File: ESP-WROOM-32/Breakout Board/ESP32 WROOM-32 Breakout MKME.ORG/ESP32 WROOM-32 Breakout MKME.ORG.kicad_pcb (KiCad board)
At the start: 2 copper layers, 5 parts, among them J1 Screw_Terminal_01x15, J2 Screw_Terminal_01x15, J3 Conn_01x15_Female, J4 Conn_01x15_Female, U1 ESP32_DevKit_V1_DOIT

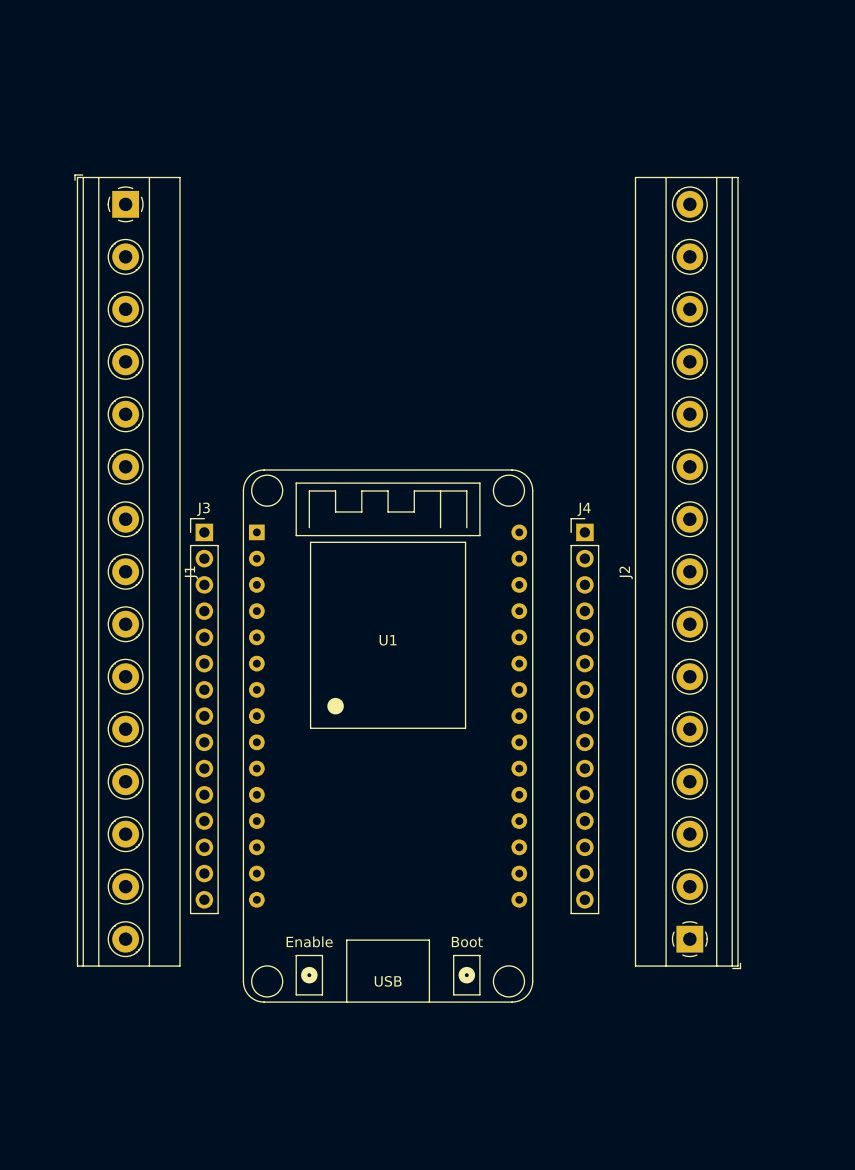
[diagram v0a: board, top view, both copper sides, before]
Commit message: Breakout board DONE
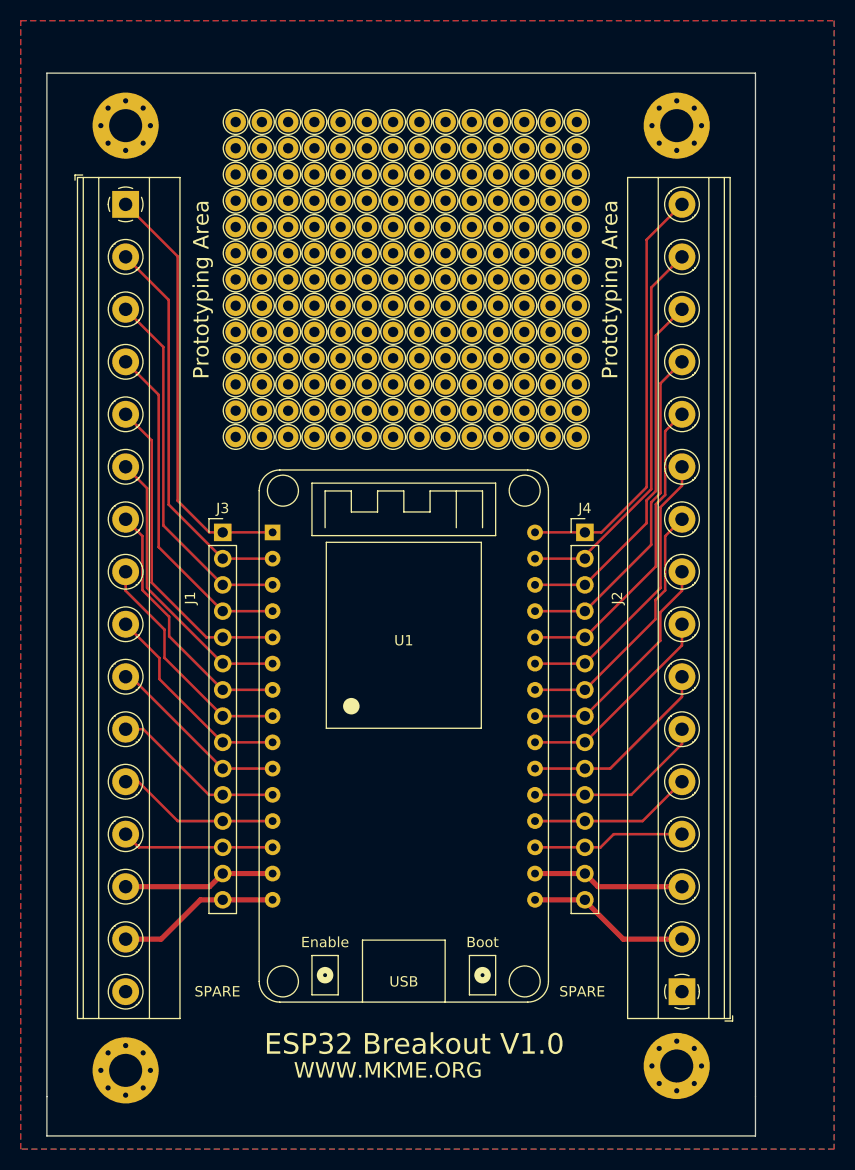
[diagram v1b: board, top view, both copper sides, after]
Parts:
- added REF**: TestPoint_THTPad_D2.0mm_Drill1.0mm, TestPoint:TestPoint_THTPad_D2.0mm_Drill1.0mm, F.Cu at (163.1, 63.1)
- added REF**: TestPoint_THTPad_D2.0mm_Drill1.0mm, TestPoint:TestPoint_THTPad_D2.0mm_Drill1.0mm, F.Cu at (140.2, 63.1)
- added REF**: TestPoint_THTPad_D2.0mm_Drill1.0mm, TestPoint:TestPoint_THTPad_D2.0mm_Drill1.0mm, F.Cu at (160.5, 45.4)
- added REF**: TestPoint_THTPad_D2.0mm_Drill1.0mm, TestPoint:TestPoint_THTPad_D2.0mm_Drill1.0mm, F.Cu at (158.0, 45.4)
- added REF**: TestPoint_THTPad_D2.0mm_Drill1.0mm, TestPoint:TestPoint_THTPad_D2.0mm_Drill1.0mm, F.Cu at (155.4, 45.4)
- added REF**: TestPoint_THTPad_D2.0mm_Drill1.0mm, TestPoint:TestPoint_THTPad_D2.0mm_Drill1.0mm, F.Cu at (152.9, 45.4)
- added REF**: TestPoint_THTPad_D2.0mm_Drill1.0mm, TestPoint:TestPoint_THTPad_D2.0mm_Drill1.0mm, F.Cu at (150.3, 45.4)
- added REF**: TestPoint_THTPad_D2.0mm_Drill1.0mm, TestPoint:TestPoint_THTPad_D2.0mm_Drill1.0mm, F.Cu at (147.8, 45.4)
- added REF**: TestPoint_THTPad_D2.0mm_Drill1.0mm, TestPoint:TestPoint_THTPad_D2.0mm_Drill1.0mm, F.Cu at (145.3, 45.4)
- added REF**: TestPoint_THTPad_D2.0mm_Drill1.0mm, TestPoint:TestPoint_THTPad_D2.0mm_Drill1.0mm, F.Cu at (142.7, 45.4)
- added REF**: TestPoint_THTPad_D2.0mm_Drill1.0mm, TestPoint:TestPoint_THTPad_D2.0mm_Drill1.0mm, F.Cu at (140.2, 45.4)
- added REF**: TestPoint_THTPad_D2.0mm_Drill1.0mm, TestPoint:TestPoint_THTPad_D2.0mm_Drill1.0mm, F.Cu at (137.7, 45.4)
- added REF**: TestPoint_THTPad_D2.0mm_Drill1.0mm, TestPoint:TestPoint_THTPad_D2.0mm_Drill1.0mm, F.Cu at (137.7, 63.1)
- added REF**: TestPoint_THTPad_D2.0mm_Drill1.0mm, TestPoint:TestPoint_THTPad_D2.0mm_Drill1.0mm, F.Cu at (135.1, 45.4)
- added REF**: TestPoint_THTPad_D2.0mm_Drill1.0mm, TestPoint:TestPoint_THTPad_D2.0mm_Drill1.0mm, F.Cu at (132.6, 45.4)
- added REF**: TestPoint_THTPad_D2.0mm_Drill1.0mm, TestPoint:TestPoint_THTPad_D2.0mm_Drill1.0mm, F.Cu at (130.0, 45.4)
- added REF**: TestPoint_THTPad_D2.0mm_Drill1.0mm, TestPoint:TestPoint_THTPad_D2.0mm_Drill1.0mm, F.Cu at (163.1, 42.8)
- added REF**: TestPoint_THTPad_D2.0mm_Drill1.0mm, TestPoint:TestPoint_THTPad_D2.0mm_Drill1.0mm, F.Cu at (160.5, 42.8)
- added REF**: TestPoint_THTPad_D2.0mm_Drill1.0mm, TestPoint:TestPoint_THTPad_D2.0mm_Drill1.0mm, F.Cu at (158.0, 42.8)
- added REF**: TestPoint_THTPad_D2.0mm_Drill1.0mm, TestPoint:TestPoint_THTPad_D2.0mm_Drill1.0mm, F.Cu at (155.4, 42.8)
- added REF**: TestPoint_THTPad_D2.0mm_Drill1.0mm, TestPoint:TestPoint_THTPad_D2.0mm_Drill1.0mm, F.Cu at (152.9, 42.8)
- added REF**: TestPoint_THTPad_D2.0mm_Drill1.0mm, TestPoint:TestPoint_THTPad_D2.0mm_Drill1.0mm, F.Cu at (150.3, 42.8)
- added REF**: TestPoint_THTPad_D2.0mm_Drill1.0mm, TestPoint:TestPoint_THTPad_D2.0mm_Drill1.0mm, F.Cu at (147.8, 42.8)
- added REF**: TestPoint_THTPad_D2.0mm_Drill1.0mm, TestPoint:TestPoint_THTPad_D2.0mm_Drill1.0mm, F.Cu at (135.1, 63.1)
- added REF**: TestPoint_THTPad_D2.0mm_Drill1.0mm, TestPoint:TestPoint_THTPad_D2.0mm_Drill1.0mm, F.Cu at (145.3, 42.8)
- added REF**: TestPoint_THTPad_D2.0mm_Drill1.0mm, TestPoint:TestPoint_THTPad_D2.0mm_Drill1.0mm, F.Cu at (142.7, 42.8)
- added REF**: TestPoint_THTPad_D2.0mm_Drill1.0mm, TestPoint:TestPoint_THTPad_D2.0mm_Drill1.0mm, F.Cu at (140.2, 42.8)
- added REF**: TestPoint_THTPad_D2.0mm_Drill1.0mm, TestPoint:TestPoint_THTPad_D2.0mm_Drill1.0mm, F.Cu at (137.7, 42.8)
- added REF**: TestPoint_THTPad_D2.0mm_Drill1.0mm, TestPoint:TestPoint_THTPad_D2.0mm_Drill1.0mm, F.Cu at (135.1, 42.8)
- added REF**: TestPoint_THTPad_D2.0mm_Drill1.0mm, TestPoint:TestPoint_THTPad_D2.0mm_Drill1.0mm, F.Cu at (132.6, 42.8)
- added REF**: TestPoint_THTPad_D2.0mm_Drill1.0mm, TestPoint:TestPoint_THTPad_D2.0mm_Drill1.0mm, F.Cu at (130.0, 42.8)
- added REF**: TestPoint_THTPad_D2.0mm_Drill1.0mm, TestPoint:TestPoint_THTPad_D2.0mm_Drill1.0mm, F.Cu at (163.1, 40.3)
- added REF**: TestPoint_THTPad_D2.0mm_Drill1.0mm, TestPoint:TestPoint_THTPad_D2.0mm_Drill1.0mm, F.Cu at (160.5, 40.3)
- added REF**: TestPoint_THTPad_D2.0mm_Drill1.0mm, TestPoint:TestPoint_THTPad_D2.0mm_Drill1.0mm, F.Cu at (158.0, 40.3)
- added REF**: TestPoint_THTPad_D2.0mm_Drill1.0mm, TestPoint:TestPoint_THTPad_D2.0mm_Drill1.0mm, F.Cu at (132.6, 63.1)
- added REF**: TestPoint_THTPad_D2.0mm_Drill1.0mm, TestPoint:TestPoint_THTPad_D2.0mm_Drill1.0mm, F.Cu at (155.4, 40.3)
- added REF**: TestPoint_THTPad_D2.0mm_Drill1.0mm, TestPoint:TestPoint_THTPad_D2.0mm_Drill1.0mm, F.Cu at (152.9, 40.3)
- added REF**: TestPoint_THTPad_D2.0mm_Drill1.0mm, TestPoint:TestPoint_THTPad_D2.0mm_Drill1.0mm, F.Cu at (150.3, 40.3)
- added REF**: TestPoint_THTPad_D2.0mm_Drill1.0mm, TestPoint:TestPoint_THTPad_D2.0mm_Drill1.0mm, F.Cu at (147.8, 40.3)
- added REF**: TestPoint_THTPad_D2.0mm_Drill1.0mm, TestPoint:TestPoint_THTPad_D2.0mm_Drill1.0mm, F.Cu at (145.3, 40.3)
- added REF**: TestPoint_THTPad_D2.0mm_Drill1.0mm, TestPoint:TestPoint_THTPad_D2.0mm_Drill1.0mm, F.Cu at (142.7, 40.3)
- added REF**: TestPoint_THTPad_D2.0mm_Drill1.0mm, TestPoint:TestPoint_THTPad_D2.0mm_Drill1.0mm, F.Cu at (140.2, 40.3)
- added REF**: TestPoint_THTPad_D2.0mm_Drill1.0mm, TestPoint:TestPoint_THTPad_D2.0mm_Drill1.0mm, F.Cu at (137.7, 40.3)
- added REF**: TestPoint_THTPad_D2.0mm_Drill1.0mm, TestPoint:TestPoint_THTPad_D2.0mm_Drill1.0mm, F.Cu at (135.1, 40.3)
- added REF**: TestPoint_THTPad_D2.0mm_Drill1.0mm, TestPoint:TestPoint_THTPad_D2.0mm_Drill1.0mm, F.Cu at (132.6, 40.3)
- added REF**: TestPoint_THTPad_D2.0mm_Drill1.0mm, TestPoint:TestPoint_THTPad_D2.0mm_Drill1.0mm, F.Cu at (130.0, 63.1)
- added REF**: TestPoint_THTPad_D2.0mm_Drill1.0mm, TestPoint:TestPoint_THTPad_D2.0mm_Drill1.0mm, F.Cu at (130.0, 40.3)
- added REF**: TestPoint_THTPad_D2.0mm_Drill1.0mm, TestPoint:TestPoint_THTPad_D2.0mm_Drill1.0mm, F.Cu at (163.1, 37.8)
- added REF**: TestPoint_THTPad_D2.0mm_Drill1.0mm, TestPoint:TestPoint_THTPad_D2.0mm_Drill1.0mm, F.Cu at (160.5, 37.8)
- added REF**: TestPoint_THTPad_D2.0mm_Drill1.0mm, TestPoint:TestPoint_THTPad_D2.0mm_Drill1.0mm, F.Cu at (158.0, 37.8)
- added REF**: TestPoint_THTPad_D2.0mm_Drill1.0mm, TestPoint:TestPoint_THTPad_D2.0mm_Drill1.0mm, F.Cu at (155.4, 37.8)
- added REF**: TestPoint_THTPad_D2.0mm_Drill1.0mm, TestPoint:TestPoint_THTPad_D2.0mm_Drill1.0mm, F.Cu at (152.9, 37.8)
- added REF**: TestPoint_THTPad_D2.0mm_Drill1.0mm, TestPoint:TestPoint_THTPad_D2.0mm_Drill1.0mm, F.Cu at (150.3, 37.8)
- added REF**: TestPoint_THTPad_D2.0mm_Drill1.0mm, TestPoint:TestPoint_THTPad_D2.0mm_Drill1.0mm, F.Cu at (147.8, 37.8)
- added REF**: TestPoint_THTPad_D2.0mm_Drill1.0mm, TestPoint:TestPoint_THTPad_D2.0mm_Drill1.0mm, F.Cu at (145.3, 37.8)
- added REF**: TestPoint_THTPad_D2.0mm_Drill1.0mm, TestPoint:TestPoint_THTPad_D2.0mm_Drill1.0mm, F.Cu at (142.7, 37.8)
- added REF**: TestPoint_THTPad_D2.0mm_Drill1.0mm, TestPoint:TestPoint_THTPad_D2.0mm_Drill1.0mm, F.Cu at (163.1, 60.6)
- added REF**: TestPoint_THTPad_D2.0mm_Drill1.0mm, TestPoint:TestPoint_THTPad_D2.0mm_Drill1.0mm, F.Cu at (140.2, 37.8)
- added REF**: TestPoint_THTPad_D2.0mm_Drill1.0mm, TestPoint:TestPoint_THTPad_D2.0mm_Drill1.0mm, F.Cu at (137.7, 37.8)
- added REF**: TestPoint_THTPad_D2.0mm_Drill1.0mm, TestPoint:TestPoint_THTPad_D2.0mm_Drill1.0mm, F.Cu at (135.1, 37.8)
- added REF**: TestPoint_THTPad_D2.0mm_Drill1.0mm, TestPoint:TestPoint_THTPad_D2.0mm_Drill1.0mm, F.Cu at (132.6, 37.8)
- added REF**: TestPoint_THTPad_D2.0mm_Drill1.0mm, TestPoint:TestPoint_THTPad_D2.0mm_Drill1.0mm, F.Cu at (130.0, 37.8)
- added REF**: TestPoint_THTPad_D2.0mm_Drill1.0mm, TestPoint:TestPoint_THTPad_D2.0mm_Drill1.0mm, F.Cu at (163.1, 35.2)
- added REF**: TestPoint_THTPad_D2.0mm_Drill1.0mm, TestPoint:TestPoint_THTPad_D2.0mm_Drill1.0mm, F.Cu at (160.5, 35.2)
- added REF**: TestPoint_THTPad_D2.0mm_Drill1.0mm, TestPoint:TestPoint_THTPad_D2.0mm_Drill1.0mm, F.Cu at (158.0, 35.2)
- added REF**: TestPoint_THTPad_D2.0mm_Drill1.0mm, TestPoint:TestPoint_THTPad_D2.0mm_Drill1.0mm, F.Cu at (155.4, 35.2)
- added REF**: TestPoint_THTPad_D2.0mm_Drill1.0mm, TestPoint:TestPoint_THTPad_D2.0mm_Drill1.0mm, F.Cu at (152.9, 35.2)
- added REF**: TestPoint_THTPad_D2.0mm_Drill1.0mm, TestPoint:TestPoint_THTPad_D2.0mm_Drill1.0mm, F.Cu at (160.5, 60.6)
- added REF**: TestPoint_THTPad_D2.0mm_Drill1.0mm, TestPoint:TestPoint_THTPad_D2.0mm_Drill1.0mm, F.Cu at (150.3, 35.2)
- added REF**: TestPoint_THTPad_D2.0mm_Drill1.0mm, TestPoint:TestPoint_THTPad_D2.0mm_Drill1.0mm, F.Cu at (147.8, 35.2)
- added REF**: TestPoint_THTPad_D2.0mm_Drill1.0mm, TestPoint:TestPoint_THTPad_D2.0mm_Drill1.0mm, F.Cu at (145.3, 35.2)
- added REF**: TestPoint_THTPad_D2.0mm_Drill1.0mm, TestPoint:TestPoint_THTPad_D2.0mm_Drill1.0mm, F.Cu at (142.7, 35.2)
- added REF**: TestPoint_THTPad_D2.0mm_Drill1.0mm, TestPoint:TestPoint_THTPad_D2.0mm_Drill1.0mm, F.Cu at (140.2, 35.2)
- added REF**: TestPoint_THTPad_D2.0mm_Drill1.0mm, TestPoint:TestPoint_THTPad_D2.0mm_Drill1.0mm, F.Cu at (137.7, 35.2)
- added REF**: TestPoint_THTPad_D2.0mm_Drill1.0mm, TestPoint:TestPoint_THTPad_D2.0mm_Drill1.0mm, F.Cu at (135.1, 35.2)
- added REF**: TestPoint_THTPad_D2.0mm_Drill1.0mm, TestPoint:TestPoint_THTPad_D2.0mm_Drill1.0mm, F.Cu at (132.6, 35.2)
- added REF**: TestPoint_THTPad_D2.0mm_Drill1.0mm, TestPoint:TestPoint_THTPad_D2.0mm_Drill1.0mm, F.Cu at (130.0, 35.2)
- added REF**: TestPoint_THTPad_D2.0mm_Drill1.0mm, TestPoint:TestPoint_THTPad_D2.0mm_Drill1.0mm, F.Cu at (163.1, 32.7)
- added REF**: TestPoint_THTPad_D2.0mm_Drill1.0mm, TestPoint:TestPoint_THTPad_D2.0mm_Drill1.0mm, F.Cu at (158.0, 60.6)
- added REF**: TestPoint_THTPad_D2.0mm_Drill1.0mm, TestPoint:TestPoint_THTPad_D2.0mm_Drill1.0mm, F.Cu at (160.5, 32.7)
- added REF**: TestPoint_THTPad_D2.0mm_Drill1.0mm, TestPoint:TestPoint_THTPad_D2.0mm_Drill1.0mm, F.Cu at (158.0, 32.7)
- added REF**: TestPoint_THTPad_D2.0mm_Drill1.0mm, TestPoint:TestPoint_THTPad_D2.0mm_Drill1.0mm, F.Cu at (155.4, 32.7)
- added REF**: TestPoint_THTPad_D2.0mm_Drill1.0mm, TestPoint:TestPoint_THTPad_D2.0mm_Drill1.0mm, F.Cu at (152.9, 32.7)
- added REF**: TestPoint_THTPad_D2.0mm_Drill1.0mm, TestPoint:TestPoint_THTPad_D2.0mm_Drill1.0mm, F.Cu at (150.3, 32.7)
- added REF**: TestPoint_THTPad_D2.0mm_Drill1.0mm, TestPoint:TestPoint_THTPad_D2.0mm_Drill1.0mm, F.Cu at (147.8, 32.7)
- added REF**: TestPoint_THTPad_D2.0mm_Drill1.0mm, TestPoint:TestPoint_THTPad_D2.0mm_Drill1.0mm, F.Cu at (145.3, 32.7)
- added REF**: TestPoint_THTPad_D2.0mm_Drill1.0mm, TestPoint:TestPoint_THTPad_D2.0mm_Drill1.0mm, F.Cu at (142.7, 32.7)
- added REF**: TestPoint_THTPad_D2.0mm_Drill1.0mm, TestPoint:TestPoint_THTPad_D2.0mm_Drill1.0mm, F.Cu at (140.2, 32.7)
- added REF**: TestPoint_THTPad_D2.0mm_Drill1.0mm, TestPoint:TestPoint_THTPad_D2.0mm_Drill1.0mm, F.Cu at (137.7, 32.7)
- added REF**: TestPoint_THTPad_D2.0mm_Drill1.0mm, TestPoint:TestPoint_THTPad_D2.0mm_Drill1.0mm, F.Cu at (155.4, 60.6)
- added REF**: TestPoint_THTPad_D2.0mm_Drill1.0mm, TestPoint:TestPoint_THTPad_D2.0mm_Drill1.0mm, F.Cu at (135.1, 32.7)
- added REF**: TestPoint_THTPad_D2.0mm_Drill1.0mm, TestPoint:TestPoint_THTPad_D2.0mm_Drill1.0mm, F.Cu at (132.6, 32.7)
- added REF**: TestPoint_THTPad_D2.0mm_Drill1.0mm, TestPoint:TestPoint_THTPad_D2.0mm_Drill1.0mm, F.Cu at (130.0, 32.7)
- added REF**: MountingHole_3.2mm_M3_Pad_Via, MountingHole:MountingHole_3.2mm_M3_Pad_Via, F.Cu at (172.7, 33.0)
- added REF**: MountingHole_3.2mm_M3_Pad_Via, MountingHole:MountingHole_3.2mm_M3_Pad_Via, F.Cu at (119.4, 33.0)
- added REF**: MountingHole_3.2mm_M3_Pad_Via, MountingHole:MountingHole_3.2mm_M3_Pad_Via, F.Cu at (119.4, 124.5)
- added REF**: MountingHole_3.2mm_M3_Pad_Via, MountingHole:MountingHole_3.2mm_M3_Pad_Via, F.Cu at (172.7, 124.0)
- added REF**: TestPoint_THTPad_D2.0mm_Drill1.0mm, TestPoint:TestPoint_THTPad_D2.0mm_Drill1.0mm, F.Cu at (152.9, 60.6)
- added REF**: TestPoint_THTPad_D2.0mm_Drill1.0mm, TestPoint:TestPoint_THTPad_D2.0mm_Drill1.0mm, F.Cu at (160.5, 63.1)
- added REF**: TestPoint_THTPad_D2.0mm_Drill1.0mm, TestPoint:TestPoint_THTPad_D2.0mm_Drill1.0mm, F.Cu at (150.3, 60.6)
- added REF**: TestPoint_THTPad_D2.0mm_Drill1.0mm, TestPoint:TestPoint_THTPad_D2.0mm_Drill1.0mm, F.Cu at (147.8, 60.6)
- added REF**: TestPoint_THTPad_D2.0mm_Drill1.0mm, TestPoint:TestPoint_THTPad_D2.0mm_Drill1.0mm, F.Cu at (145.3, 60.6)
- added REF**: TestPoint_THTPad_D2.0mm_Drill1.0mm, TestPoint:TestPoint_THTPad_D2.0mm_Drill1.0mm, F.Cu at (142.7, 60.6)
- added REF**: TestPoint_THTPad_D2.0mm_Drill1.0mm, TestPoint:TestPoint_THTPad_D2.0mm_Drill1.0mm, F.Cu at (140.2, 60.6)
- added REF**: TestPoint_THTPad_D2.0mm_Drill1.0mm, TestPoint:TestPoint_THTPad_D2.0mm_Drill1.0mm, F.Cu at (137.7, 60.6)
- added REF**: TestPoint_THTPad_D2.0mm_Drill1.0mm, TestPoint:TestPoint_THTPad_D2.0mm_Drill1.0mm, F.Cu at (135.1, 60.6)
- added REF**: TestPoint_THTPad_D2.0mm_Drill1.0mm, TestPoint:TestPoint_THTPad_D2.0mm_Drill1.0mm, F.Cu at (132.6, 60.6)
- added REF**: TestPoint_THTPad_D2.0mm_Drill1.0mm, TestPoint:TestPoint_THTPad_D2.0mm_Drill1.0mm, F.Cu at (130.0, 60.6)
- added REF**: TestPoint_THTPad_D2.0mm_Drill1.0mm, TestPoint:TestPoint_THTPad_D2.0mm_Drill1.0mm, F.Cu at (163.1, 58.1)
- added REF**: TestPoint_THTPad_D2.0mm_Drill1.0mm, TestPoint:TestPoint_THTPad_D2.0mm_Drill1.0mm, F.Cu at (158.0, 63.1)
- added REF**: TestPoint_THTPad_D2.0mm_Drill1.0mm, TestPoint:TestPoint_THTPad_D2.0mm_Drill1.0mm, F.Cu at (160.5, 58.1)
- added REF**: TestPoint_THTPad_D2.0mm_Drill1.0mm, TestPoint:TestPoint_THTPad_D2.0mm_Drill1.0mm, F.Cu at (158.0, 58.1)
- added REF**: TestPoint_THTPad_D2.0mm_Drill1.0mm, TestPoint:TestPoint_THTPad_D2.0mm_Drill1.0mm, F.Cu at (155.4, 58.1)
- added REF**: TestPoint_THTPad_D2.0mm_Drill1.0mm, TestPoint:TestPoint_THTPad_D2.0mm_Drill1.0mm, F.Cu at (152.9, 58.1)
- added REF**: TestPoint_THTPad_D2.0mm_Drill1.0mm, TestPoint:TestPoint_THTPad_D2.0mm_Drill1.0mm, F.Cu at (150.3, 58.1)
- added REF**: TestPoint_THTPad_D2.0mm_Drill1.0mm, TestPoint:TestPoint_THTPad_D2.0mm_Drill1.0mm, F.Cu at (147.8, 58.1)
- added REF**: TestPoint_THTPad_D2.0mm_Drill1.0mm, TestPoint:TestPoint_THTPad_D2.0mm_Drill1.0mm, F.Cu at (145.3, 58.1)
- added REF**: TestPoint_THTPad_D2.0mm_Drill1.0mm, TestPoint:TestPoint_THTPad_D2.0mm_Drill1.0mm, F.Cu at (142.7, 58.1)
- added REF**: TestPoint_THTPad_D2.0mm_Drill1.0mm, TestPoint:TestPoint_THTPad_D2.0mm_Drill1.0mm, F.Cu at (140.2, 58.1)
- added REF**: TestPoint_THTPad_D2.0mm_Drill1.0mm, TestPoint:TestPoint_THTPad_D2.0mm_Drill1.0mm, F.Cu at (137.7, 58.1)
- added REF**: TestPoint_THTPad_D2.0mm_Drill1.0mm, TestPoint:TestPoint_THTPad_D2.0mm_Drill1.0mm, F.Cu at (155.4, 63.1)
- added REF**: TestPoint_THTPad_D2.0mm_Drill1.0mm, TestPoint:TestPoint_THTPad_D2.0mm_Drill1.0mm, F.Cu at (135.1, 58.1)
- added REF**: TestPoint_THTPad_D2.0mm_Drill1.0mm, TestPoint:TestPoint_THTPad_D2.0mm_Drill1.0mm, F.Cu at (132.6, 58.1)
- added REF**: TestPoint_THTPad_D2.0mm_Drill1.0mm, TestPoint:TestPoint_THTPad_D2.0mm_Drill1.0mm, F.Cu at (130.0, 58.1)
- added REF**: TestPoint_THTPad_D2.0mm_Drill1.0mm, TestPoint:TestPoint_THTPad_D2.0mm_Drill1.0mm, F.Cu at (163.1, 55.5)
- added REF**: TestPoint_THTPad_D2.0mm_Drill1.0mm, TestPoint:TestPoint_THTPad_D2.0mm_Drill1.0mm, F.Cu at (160.5, 55.5)
- added REF**: TestPoint_THTPad_D2.0mm_Drill1.0mm, TestPoint:TestPoint_THTPad_D2.0mm_Drill1.0mm, F.Cu at (158.0, 55.5)
- added REF**: TestPoint_THTPad_D2.0mm_Drill1.0mm, TestPoint:TestPoint_THTPad_D2.0mm_Drill1.0mm, F.Cu at (155.4, 55.5)
- added REF**: TestPoint_THTPad_D2.0mm_Drill1.0mm, TestPoint:TestPoint_THTPad_D2.0mm_Drill1.0mm, F.Cu at (152.9, 55.5)
- added REF**: TestPoint_THTPad_D2.0mm_Drill1.0mm, TestPoint:TestPoint_THTPad_D2.0mm_Drill1.0mm, F.Cu at (150.3, 55.5)
- added REF**: TestPoint_THTPad_D2.0mm_Drill1.0mm, TestPoint:TestPoint_THTPad_D2.0mm_Drill1.0mm, F.Cu at (147.8, 55.5)
- added REF**: TestPoint_THTPad_D2.0mm_Drill1.0mm, TestPoint:TestPoint_THTPad_D2.0mm_Drill1.0mm, F.Cu at (152.9, 63.1)
- added REF**: TestPoint_THTPad_D2.0mm_Drill1.0mm, TestPoint:TestPoint_THTPad_D2.0mm_Drill1.0mm, F.Cu at (145.3, 55.5)
- added REF**: TestPoint_THTPad_D2.0mm_Drill1.0mm, TestPoint:TestPoint_THTPad_D2.0mm_Drill1.0mm, F.Cu at (142.7, 55.5)
- added REF**: TestPoint_THTPad_D2.0mm_Drill1.0mm, TestPoint:TestPoint_THTPad_D2.0mm_Drill1.0mm, F.Cu at (140.2, 55.5)
- added REF**: TestPoint_THTPad_D2.0mm_Drill1.0mm, TestPoint:TestPoint_THTPad_D2.0mm_Drill1.0mm, F.Cu at (137.7, 55.5)
- added REF**: TestPoint_THTPad_D2.0mm_Drill1.0mm, TestPoint:TestPoint_THTPad_D2.0mm_Drill1.0mm, F.Cu at (135.1, 55.5)
- added REF**: TestPoint_THTPad_D2.0mm_Drill1.0mm, TestPoint:TestPoint_THTPad_D2.0mm_Drill1.0mm, F.Cu at (132.6, 55.5)
- added REF**: TestPoint_THTPad_D2.0mm_Drill1.0mm, TestPoint:TestPoint_THTPad_D2.0mm_Drill1.0mm, F.Cu at (130.0, 55.5)
- added REF**: TestPoint_THTPad_D2.0mm_Drill1.0mm, TestPoint:TestPoint_THTPad_D2.0mm_Drill1.0mm, F.Cu at (163.1, 53.0)
- added REF**: TestPoint_THTPad_D2.0mm_Drill1.0mm, TestPoint:TestPoint_THTPad_D2.0mm_Drill1.0mm, F.Cu at (160.5, 53.0)
- added REF**: TestPoint_THTPad_D2.0mm_Drill1.0mm, TestPoint:TestPoint_THTPad_D2.0mm_Drill1.0mm, F.Cu at (158.0, 53.0)
- added REF**: TestPoint_THTPad_D2.0mm_Drill1.0mm, TestPoint:TestPoint_THTPad_D2.0mm_Drill1.0mm, F.Cu at (150.3, 63.1)
- added REF**: TestPoint_THTPad_D2.0mm_Drill1.0mm, TestPoint:TestPoint_THTPad_D2.0mm_Drill1.0mm, F.Cu at (155.4, 53.0)
- added REF**: TestPoint_THTPad_D2.0mm_Drill1.0mm, TestPoint:TestPoint_THTPad_D2.0mm_Drill1.0mm, F.Cu at (152.9, 53.0)
- added REF**: TestPoint_THTPad_D2.0mm_Drill1.0mm, TestPoint:TestPoint_THTPad_D2.0mm_Drill1.0mm, F.Cu at (150.3, 53.0)
- added REF**: TestPoint_THTPad_D2.0mm_Drill1.0mm, TestPoint:TestPoint_THTPad_D2.0mm_Drill1.0mm, F.Cu at (147.8, 53.0)
- added REF**: TestPoint_THTPad_D2.0mm_Drill1.0mm, TestPoint:TestPoint_THTPad_D2.0mm_Drill1.0mm, F.Cu at (145.3, 53.0)
- added REF**: TestPoint_THTPad_D2.0mm_Drill1.0mm, TestPoint:TestPoint_THTPad_D2.0mm_Drill1.0mm, F.Cu at (142.7, 53.0)
- added REF**: TestPoint_THTPad_D2.0mm_Drill1.0mm, TestPoint:TestPoint_THTPad_D2.0mm_Drill1.0mm, F.Cu at (140.2, 53.0)
- added REF**: TestPoint_THTPad_D2.0mm_Drill1.0mm, TestPoint:TestPoint_THTPad_D2.0mm_Drill1.0mm, F.Cu at (137.7, 53.0)
- added REF**: TestPoint_THTPad_D2.0mm_Drill1.0mm, TestPoint:TestPoint_THTPad_D2.0mm_Drill1.0mm, F.Cu at (135.1, 53.0)
- added REF**: TestPoint_THTPad_D2.0mm_Drill1.0mm, TestPoint:TestPoint_THTPad_D2.0mm_Drill1.0mm, F.Cu at (132.6, 53.0)
- added REF**: TestPoint_THTPad_D2.0mm_Drill1.0mm, TestPoint:TestPoint_THTPad_D2.0mm_Drill1.0mm, F.Cu at (147.8, 63.1)
- added REF**: TestPoint_THTPad_D2.0mm_Drill1.0mm, TestPoint:TestPoint_THTPad_D2.0mm_Drill1.0mm, F.Cu at (130.0, 53.0)
- added REF**: TestPoint_THTPad_D2.0mm_Drill1.0mm, TestPoint:TestPoint_THTPad_D2.0mm_Drill1.0mm, F.Cu at (163.1, 50.5)
- added REF**: TestPoint_THTPad_D2.0mm_Drill1.0mm, TestPoint:TestPoint_THTPad_D2.0mm_Drill1.0mm, F.Cu at (160.5, 50.5)
- added REF**: TestPoint_THTPad_D2.0mm_Drill1.0mm, TestPoint:TestPoint_THTPad_D2.0mm_Drill1.0mm, F.Cu at (158.0, 50.5)
- added REF**: TestPoint_THTPad_D2.0mm_Drill1.0mm, TestPoint:TestPoint_THTPad_D2.0mm_Drill1.0mm, F.Cu at (155.4, 50.5)
- added REF**: TestPoint_THTPad_D2.0mm_Drill1.0mm, TestPoint:TestPoint_THTPad_D2.0mm_Drill1.0mm, F.Cu at (152.9, 50.5)
- added REF**: TestPoint_THTPad_D2.0mm_Drill1.0mm, TestPoint:TestPoint_THTPad_D2.0mm_Drill1.0mm, F.Cu at (150.3, 50.5)
- added REF**: TestPoint_THTPad_D2.0mm_Drill1.0mm, TestPoint:TestPoint_THTPad_D2.0mm_Drill1.0mm, F.Cu at (147.8, 50.5)
- added REF**: TestPoint_THTPad_D2.0mm_Drill1.0mm, TestPoint:TestPoint_THTPad_D2.0mm_Drill1.0mm, F.Cu at (145.3, 50.5)
- added REF**: TestPoint_THTPad_D2.0mm_Drill1.0mm, TestPoint:TestPoint_THTPad_D2.0mm_Drill1.0mm, F.Cu at (142.7, 50.5)
- added REF**: TestPoint_THTPad_D2.0mm_Drill1.0mm, TestPoint:TestPoint_THTPad_D2.0mm_Drill1.0mm, F.Cu at (145.3, 63.1)
- added REF**: TestPoint_THTPad_D2.0mm_Drill1.0mm, TestPoint:TestPoint_THTPad_D2.0mm_Drill1.0mm, F.Cu at (140.2, 50.5)
- added REF**: TestPoint_THTPad_D2.0mm_Drill1.0mm, TestPoint:TestPoint_THTPad_D2.0mm_Drill1.0mm, F.Cu at (137.7, 50.5)
- added REF**: TestPoint_THTPad_D2.0mm_Drill1.0mm, TestPoint:TestPoint_THTPad_D2.0mm_Drill1.0mm, F.Cu at (135.1, 50.5)
- added REF**: TestPoint_THTPad_D2.0mm_Drill1.0mm, TestPoint:TestPoint_THTPad_D2.0mm_Drill1.0mm, F.Cu at (132.6, 50.5)
- added REF**: TestPoint_THTPad_D2.0mm_Drill1.0mm, TestPoint:TestPoint_THTPad_D2.0mm_Drill1.0mm, F.Cu at (130.0, 50.5)
- added REF**: TestPoint_THTPad_D2.0mm_Drill1.0mm, TestPoint:TestPoint_THTPad_D2.0mm_Drill1.0mm, F.Cu at (163.1, 47.9)
- added REF**: TestPoint_THTPad_D2.0mm_Drill1.0mm, TestPoint:TestPoint_THTPad_D2.0mm_Drill1.0mm, F.Cu at (160.5, 47.9)
- added REF**: TestPoint_THTPad_D2.0mm_Drill1.0mm, TestPoint:TestPoint_THTPad_D2.0mm_Drill1.0mm, F.Cu at (158.0, 47.9)
- added REF**: TestPoint_THTPad_D2.0mm_Drill1.0mm, TestPoint:TestPoint_THTPad_D2.0mm_Drill1.0mm, F.Cu at (155.4, 47.9)
- added REF**: TestPoint_THTPad_D2.0mm_Drill1.0mm, TestPoint:TestPoint_THTPad_D2.0mm_Drill1.0mm, F.Cu at (152.9, 47.9)
- added REF**: TestPoint_THTPad_D2.0mm_Drill1.0mm, TestPoint:TestPoint_THTPad_D2.0mm_Drill1.0mm, F.Cu at (142.7, 63.1)
- added REF**: TestPoint_THTPad_D2.0mm_Drill1.0mm, TestPoint:TestPoint_THTPad_D2.0mm_Drill1.0mm, F.Cu at (150.3, 47.9)
- added REF**: TestPoint_THTPad_D2.0mm_Drill1.0mm, TestPoint:TestPoint_THTPad_D2.0mm_Drill1.0mm, F.Cu at (147.8, 47.9)
- added REF**: TestPoint_THTPad_D2.0mm_Drill1.0mm, TestPoint:TestPoint_THTPad_D2.0mm_Drill1.0mm, F.Cu at (145.3, 47.9)
- added REF**: TestPoint_THTPad_D2.0mm_Drill1.0mm, TestPoint:TestPoint_THTPad_D2.0mm_Drill1.0mm, F.Cu at (142.7, 47.9)
- added REF**: TestPoint_THTPad_D2.0mm_Drill1.0mm, TestPoint:TestPoint_THTPad_D2.0mm_Drill1.0mm, F.Cu at (140.2, 47.9)
- added REF**: TestPoint_THTPad_D2.0mm_Drill1.0mm, TestPoint:TestPoint_THTPad_D2.0mm_Drill1.0mm, F.Cu at (137.7, 47.9)
- added REF**: TestPoint_THTPad_D2.0mm_Drill1.0mm, TestPoint:TestPoint_THTPad_D2.0mm_Drill1.0mm, F.Cu at (135.1, 47.9)
- added REF**: TestPoint_THTPad_D2.0mm_Drill1.0mm, TestPoint:TestPoint_THTPad_D2.0mm_Drill1.0mm, F.Cu at (132.6, 47.9)
- added REF**: TestPoint_THTPad_D2.0mm_Drill1.0mm, TestPoint:TestPoint_THTPad_D2.0mm_Drill1.0mm, F.Cu at (130.0, 47.9)
- added REF**: TestPoint_THTPad_D2.0mm_Drill1.0mm, TestPoint:TestPoint_THTPad_D2.0mm_Drill1.0mm, F.Cu at (163.1, 45.4)
- J1, J2: footprint TerminalBlock_Phoenix:TerminalBlock_Phoenix_MKDS-1,5-15-5.08_1x15_P5.08mm_Horizontal -> TerminalBlock_Phoenix:TerminalBlock_Phoenix_MKDS-1,5-16-5.08_1x16_P5.08mm_Horizontal
- moved J2 5.14 mm to (173.2, 116.8)
- moved J3 1.78 mm to (128.8, 72.4)
- moved U1 1.52 mm to (146.3, 72.4)
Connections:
- J2 pad 1: 3V3 -> Net-(J2-Pad1)
- J2 pad 10: D19 -> D18
- J2 pad 11: D21 -> D19
- J2 pad 12: RX0 -> D21
- J2 pad 13: TX0 -> RX0
- J2 pad 14: D22 -> TX0
- J2 pad 15: D23 -> D22
- J2 pad 2: GND -> 3V3
- J2 pad 3: D15 -> GND
- J2 pad 4: D2 -> D15
- J2 pad 5: D4 -> D2
- J2 pad 6: RX2 -> D4
- J2 pad 7: TX2 -> RX2
- J2 pad 8: D5 -> TX2
- J2 pad 9: D18 -> D5
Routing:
- net D23: track 0.00 -> 42.2 mm
- net EN: track 0.00 -> 41.2 mm
- net VP: track 0.00 -> 37.9 mm
- net D22: track 0.00 -> 37.9 mm
- net VN: track 0.00 -> 35.4 mm
- net TX0: track 0.00 -> 35.4 mm
- net RX0: track 0.00 -> 33.2 mm
- net D34: track 0.00 -> 32.8 mm
- net D35: track 0.00 -> 31.2 mm
- net D21: track 0.00 -> 30.4 mm
- net GND: track 0.00 -> 29.5 mm
- net D32: track 0.00 -> 27.8 mm
- net D19: track 0.00 -> 27.8 mm
- net D18: track 0.00 -> 25.2 mm
- net D33: track 0.00 -> 25.2 mm
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- added copper zone on B.Cu, net GND
- added copper zone on F.Cu, net GND
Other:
- board outline added: 68.6 x 102.9 mm
- board text added: "3V3"
- board text added: "D12"
- board text added: "D13"
- board text added: "D14"
- board text added: "D15"
- board text added: "D18"
- board text added: "D19"
- board text added: "D2"
- board text added: "D21"
- board text added: "D22"
- board text added: "D23"
- board text added: "D25"
- board text added: "D26"
- board text added: "D27"
- board text added: "D32"
- board text added: "D33"
- board text added: "D34"
- board text added: "D35"
- board text added: "D4"
- board text added: "D5"
- board text added: "EN"
- board text added: "ESP32 Breakout Dev Board www.mkme.org YouTube.com/mkmeorg"
- board text added: "ESP32 Breakout V1.0"
- board text added: "GND"
- board text added: "Prototyping Area"
- board text added: "RX0"
- board text added: "RX2"
- board text added: "SPARE"
- board text added: "TX0"
- board text added: "TX2"
- board text added: "VIN"
- board text added: "VN"
- board text added: "VP"
- board text added: "WWW.MKME.ORG"
